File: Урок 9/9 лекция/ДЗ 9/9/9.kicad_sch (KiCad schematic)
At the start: 11 parts, among them IC1 LM393P, SW1 SW_Push

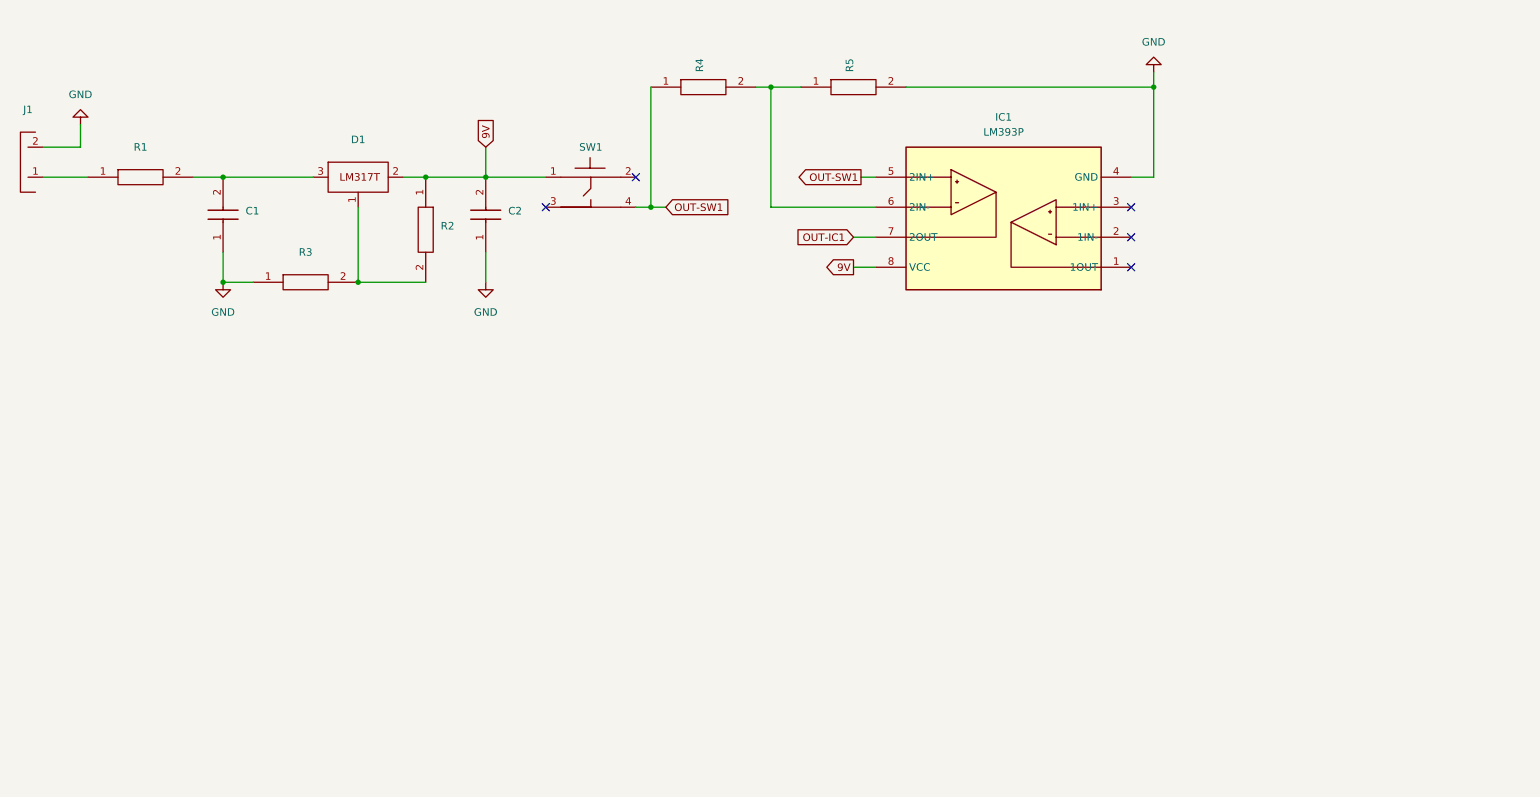
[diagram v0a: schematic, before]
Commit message: 1
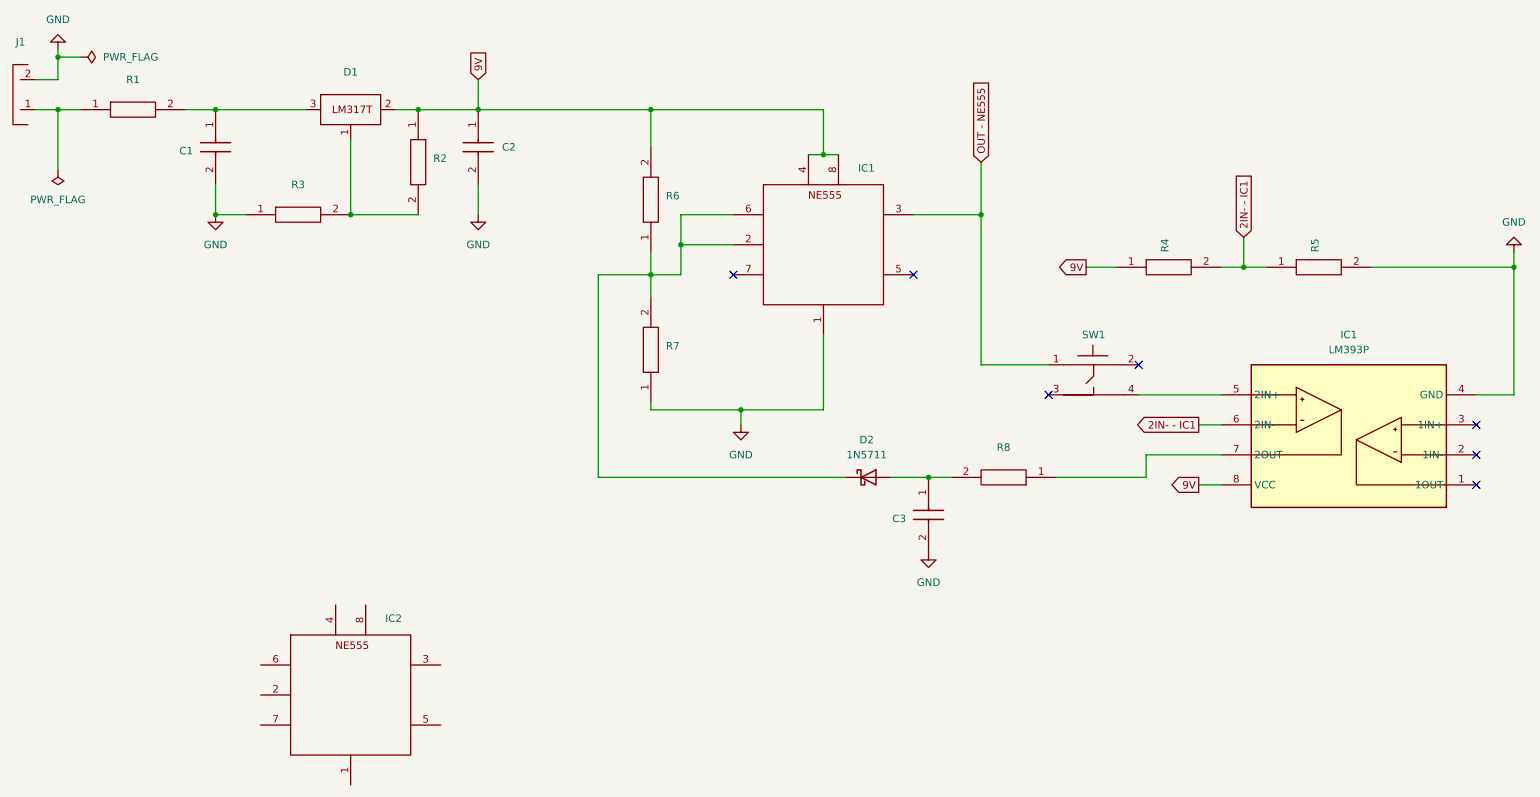
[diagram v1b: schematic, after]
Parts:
- removed C1: ~, My_lib2:564R60GAD10, symbol My_lib2:C_564R60GAD10
- added C2, C3: ~, My_lib2:C - 564R60GAD10, symbol My_lib2:C_564R60GAD10
- added D2: 1N5711, Diode_THT:D_DO-35_SOD27_P7.62mm_Horizontal, symbol Diode:1N5711
- added IC1, IC2: ~, My_lib2:8-DIP, symbol My_lib2:NE555
- added R6, R7, R8: ~, My_lib2:R axil, symbol My_lib2:R_CF100-3K3-J-TB-070-62
- C1: renamed from C2; footprint My_lib2:564R60GAD10 -> My_lib2:C - 564R60GAD10
- R1, R2, R3, R4, R5: footprint My_lib2:R -> My_lib2:R axil
- SW1: footprint My_lib2:0650HIM-130G-G -> My_lib2:SW - 0650HIM-130G-G
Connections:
- net 9V: now also R4.1, C2.1, IC1.4, IC1.8, R6.2; no longer C1.2, SW1.1
- net GND: now also C1.2, C2.2, C3.2, IC1.1, R7.1; no longer C1.1
- net 2IN- - IC1: now reaches IC1.6 (2IN-), R4.2, R5.1
- net at D1.3, R1.2: now also C1.1
- net OUT-IC1: no longer names the net of IC1.7 (2OUT)
- net OUT-IC1: now also R8.1
- net OUT-SW1: no longer names the net of IC1.5 (2IN+), SW1.4 (2)
- net OUT-SW1: no longer R4.1
- new net: D2.1 (K), IC1.2, IC1.6, R6.1, R7.2
- new net: C3.1, D2.2 (A), R8.2
- new net OUT - NE555: IC1.3, SW1.1
- no-connect marks 5 -> 7
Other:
- moved on the sheet: C1, D1, IC1, J1, R1, R2, R3, R4, R5, SW1
